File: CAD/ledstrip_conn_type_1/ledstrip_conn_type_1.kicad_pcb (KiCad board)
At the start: 2 copper layers, 22.3 x 19.3 mm, 4 parts, among them J1 led_strip_output, J2 led_strip_input, J3 led_strip_input, J4 Conn_01x03

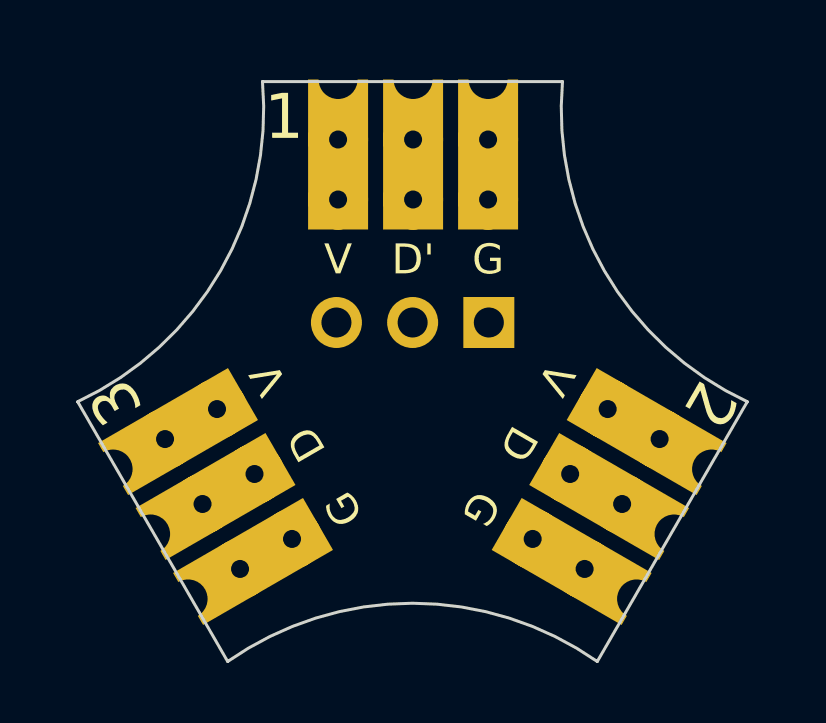
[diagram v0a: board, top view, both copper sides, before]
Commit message: feat: added wires to pcb
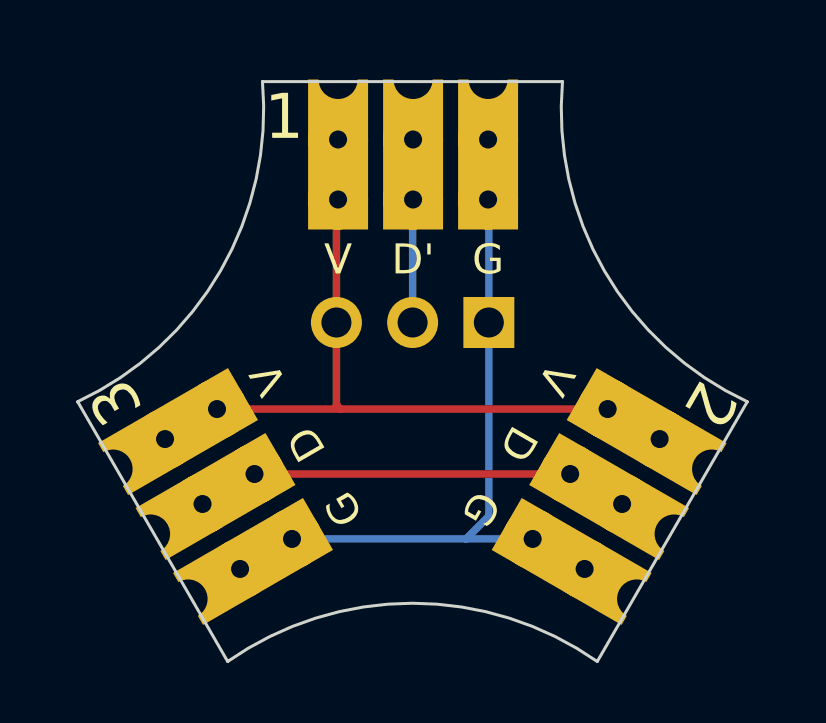
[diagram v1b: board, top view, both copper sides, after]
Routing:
- net /G: track 0.00 -> 35.4 mm
- net /V: track 0.00 -> 32.1 mm
- net /D: track 0.00 -> 18.6 mm
- net /D': track 0.00 -> 11.7 mm
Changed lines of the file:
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@@
     (effects (font (size 1.5 1.5) (thickness 0.3)))
   )
+  (segment (start 151.285898 110.134936) (end 142.384936 110.134936) (width 0.25) (layer "F.Cu") (net 1))
+  (segment (start 142.384936 110.134936) (end 142.245 109.995) (width 0.25) (layer "F.Cu") (net 1))
+  (segment (start 142.245 99.4) (end 142.3 99.345) (width 0.25) (layer "F.Cu") (net 1))
+  (segment (start 142.245 107.25) (end 142.245 103.205) (width 0.25) (layer "F.Cu") (net 1))
+  (segment (start 153.177431 112.026469) (end 154.562135 112.026469) (width 0.25) (layer "F.Cu") (net 1))
+  (segment (start 142.3 103.15) (end 142.3 99.345) (width 0.25) (layer "F.Cu") (net 1))
+  (segment (start 151.285898 110.134936) (end 153.177431 112.026469) (width 0.25) (layer "F.Cu") (net 1))
+  (segment (start 142.245 103.205) (end 142.3 103.15) (width 0.25) (layer "F.Cu") (net 1))
+  (segment (start 142.384936 110.134936) (end 138.264102 110.134936) (width 0.25) (layer "F.Cu") (net 1))
+  (segment (start 136.3769 112.022138) (end 134.995366 112.022138) (width 0.25) (layer "F.Cu") (net 1))
+  (segment (start 142.245 109.995) (end 142.245 107.25) (width 0.25) (layer "F.Cu") (net 1))
+  (segment (start 138.264102 110.134936) (end 136.3769 112.022138) (width 0.25) (layer "F.Cu") (net 1))
+  (segment (start 150.035898 112.3) (end 151.927415 114.191517) (width 0.25) (layer "F.Cu") (net 2))
+  (segment (start 139.514102 112.3) (end 137.626915 114.187187) (width 0.25) (layer "F.Cu") (net 2))
+  (segment (start 150.035898 112.3) (end 139.514102 112.3) (width 0.25) (layer "F.Cu") (net 2))
+  (segment (start 151.927415 114.191517) (end 153.312108 114.191517) (width 0.25) (layer "F.Cu") (net 2))
+  (segment (start 137.626915 114.187187) (end 136.245393 114.187187) (width 0.25) (layer "F.Cu") (net 2))
+  (segment (start 147.325 99.37) (end 147.3 99.345) (width 0.25) (layer "F.Cu") (net 3))
+  (segment (start 146.565064 114.465064) (end 147.325 113.705128) (width 0.25) (layer "B.Cu") (net 3))
+  (segment (start 148.785898 114.465064) (end 150.677399 116.356565) (width 0.25) (layer "B.Cu") (net 3))
+  (segment (start 150.677399 116.356565) (end 152.062079 116.356565) (width 0.25) (layer "B.Cu") (net 3))
+  (segment (start 147.325 113.705128) (end 147.325 107.25) (width 0.25) (layer "B.Cu") (net 3))
+  (segment (start 138.723855 116.505311) (end 137.583802 116.505311) (width 0.25) (layer "B.Cu") (net 3))
+  (segment (start 147.3 103.15) (end 147.3 99.345) (width 0.25) (layer "B.Cu") (net 3))
+  (segment (start 147.325 107.25) (end 147.325 99.37) (width 0.25) (layer "B.Cu") (net 3))
+  (segment (start 148.785898 114.465064) (end 146.565064 114.465064) (width 0.25) (layer "B.Cu") (net 3))
+  (segment (start 146.565064 114.465064) (end 140.764102 114.465064) (width 0.25) (layer "B.Cu") (net 3))
+  (segment (start 138.723855 116.505311) (end 140.764102 114.465064) (width 0.25) (layer "B.Cu") (net 3))
+  (segment (start 144.785 99.36) (end 144.8 99.345) (width 0.25) (layer "F.Cu") (net 4))
+  (segment (start 144.785 107.25) (end 144.785 99.36) (width 0.25) (layer "B.Cu") (net 4))
+  (segment (start 144.8 103.15) (end 144.8 99.345) (width 0.25) (layer "B.Cu") (net 4))
 )
